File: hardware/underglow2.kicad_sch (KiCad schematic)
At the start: 1 part, among them J101 J_Delphi_Sicma_24

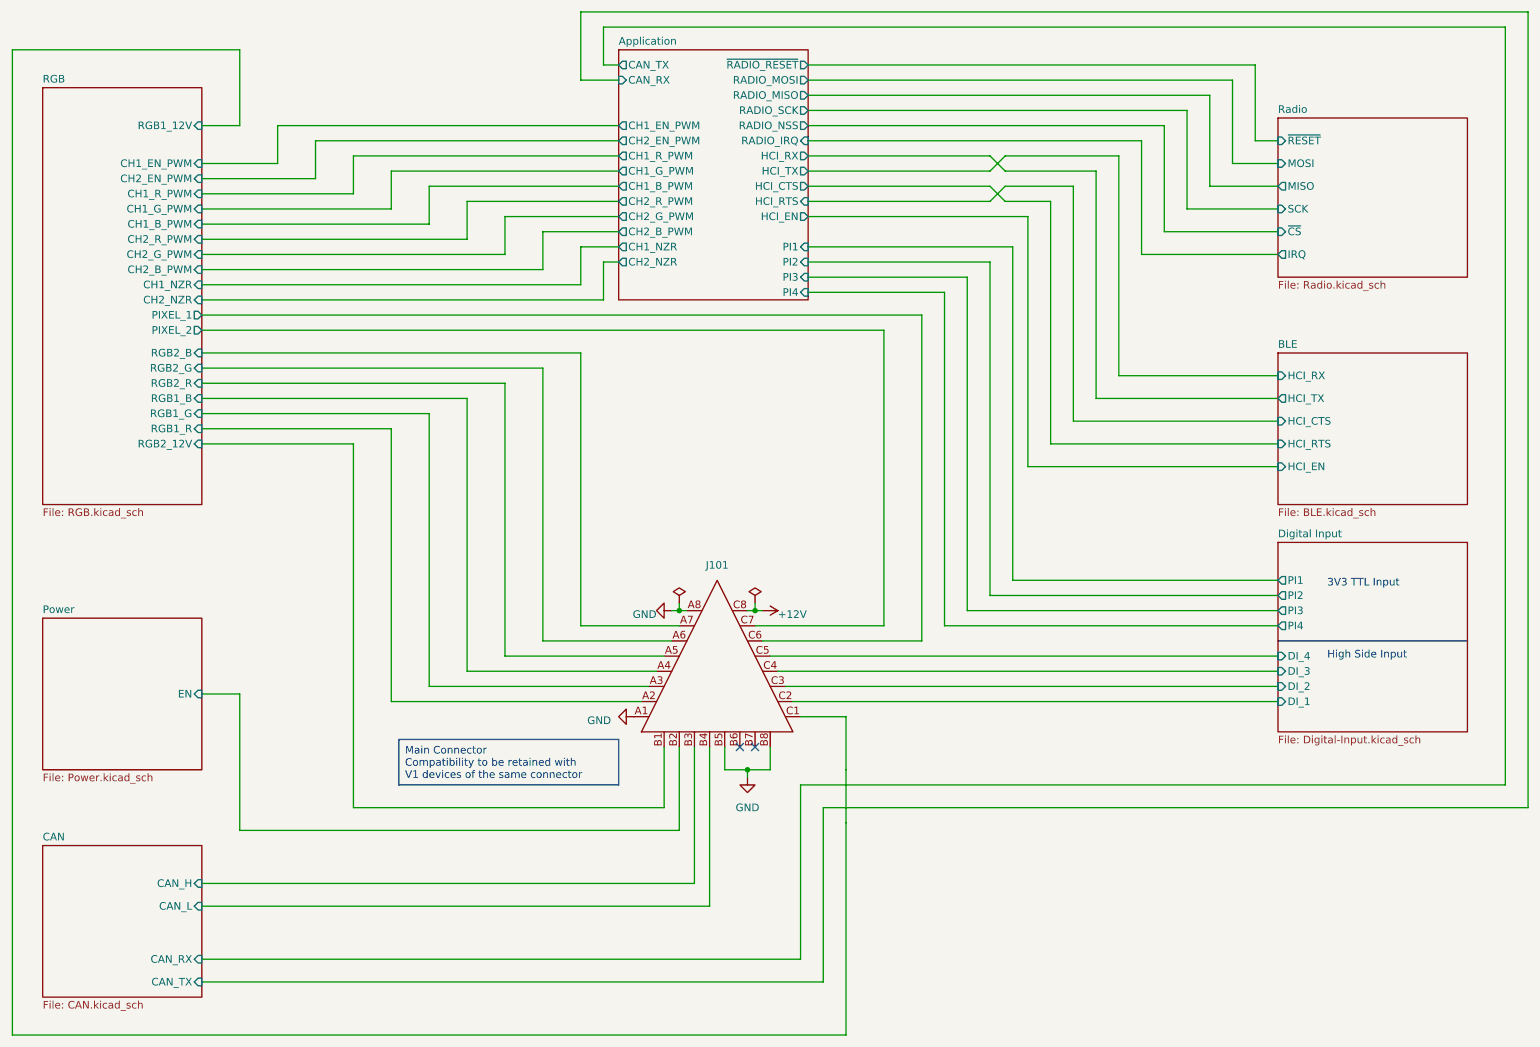
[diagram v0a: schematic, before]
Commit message: ughhhhhhhhhhhhhhhhhhhhhhhhhhhhhhhhhhhhhhhhhhhhhhhhhhh
Signed-off-by: Connor Rigby <connorr@hey.com>
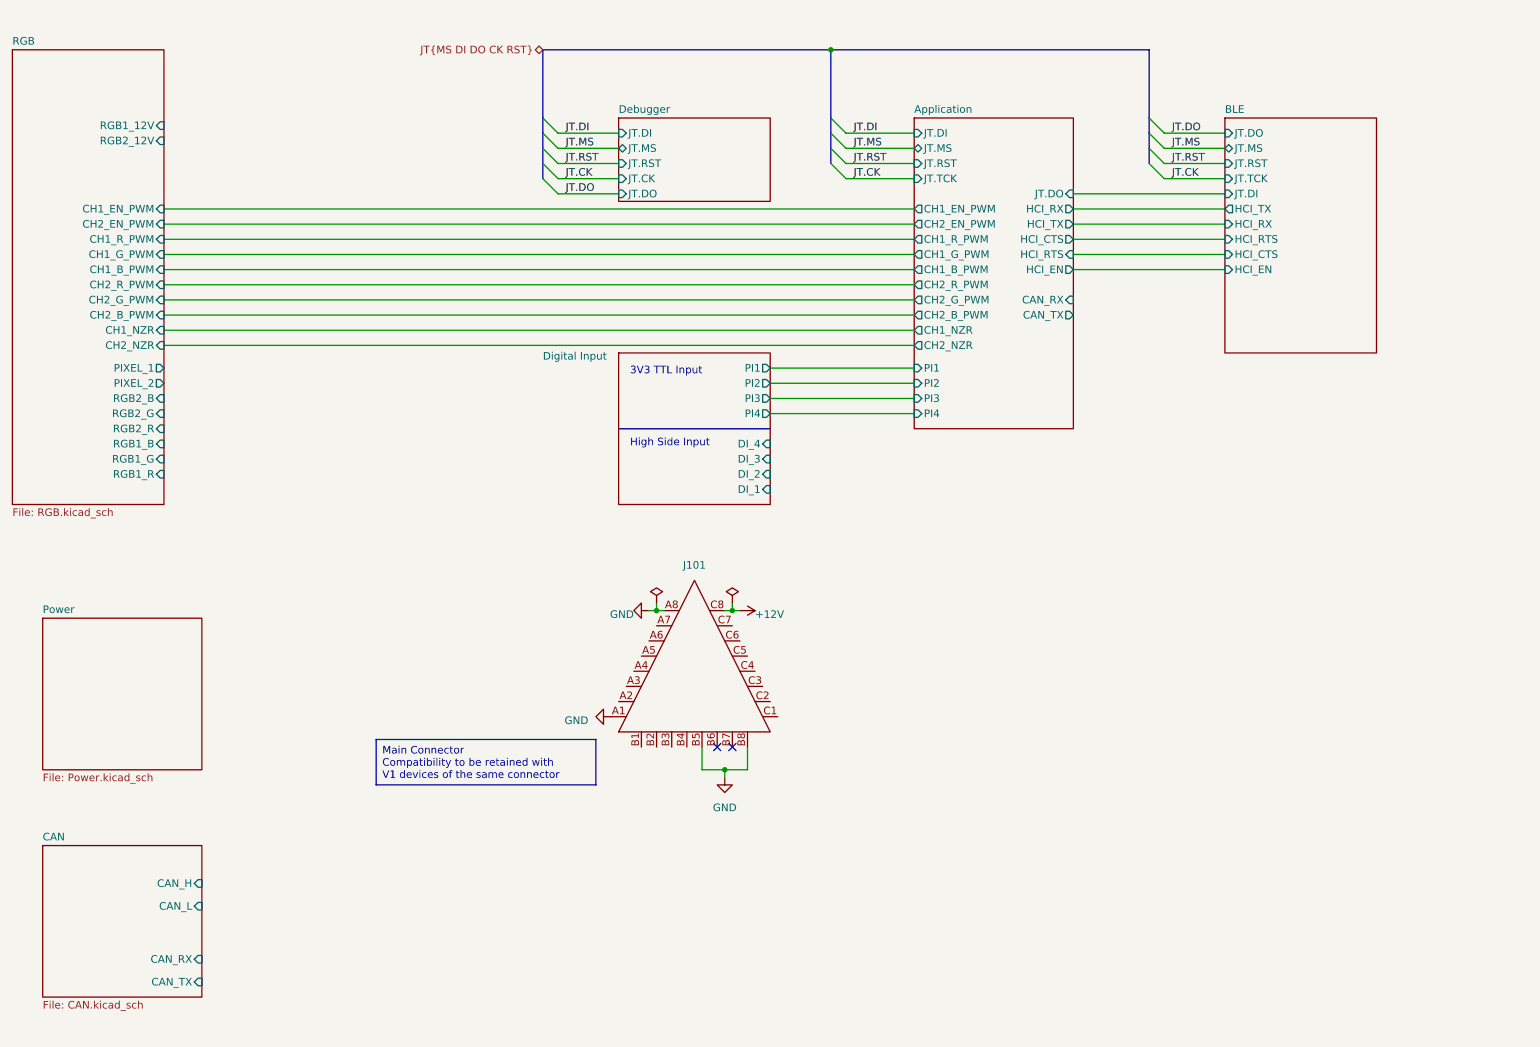
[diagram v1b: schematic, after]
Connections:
- net CAN/CAN_H: no longer J101.B3
- net CAN/CAN_L: no longer J101.B4
- net Digital Input/DI_1: no longer J101.C2
- net Digital Input/DI_2: no longer J101.C3
- net Digital Input/DI_3: no longer J101.C4
- net Digital Input/DI_4: no longer J101.C5
- net RGB/PIXEL_1: no longer J101.C6
- net RGB/PIXEL_2: no longer J101.C7
- net RGB/RGB1_12V: no longer J101.C1
- net RGB/RGB1_B: no longer J101.A4
- net RGB/RGB1_G: no longer J101.A3
- net RGB/RGB1_R: no longer J101.A2
- net RGB/RGB2_12V: no longer J101.B1
- net RGB/RGB2_B: no longer J101.A7
- net RGB/RGB2_G: no longer J101.A6
- net RGB/RGB2_R: no longer J101.A5
- net Power/EN: no longer names the net of J101.B2
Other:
- removed sheet Radio
- added sheet Debugger (Debugger.kicad_sch)
- sheet Application ports: added JT.DI, JT.DO, JT.MS, JT.RST, JT.TCK; removed RADIO_IRQ, RADIO_MISO, RADIO_MOSI, RADIO_NSS, RADIO_SCK, ~{RADIO_RESET}
- sheet BLE ports: added JT.DI, JT.DO, JT.MS, JT.RST, JT.TCK; removed none
- sheet Power ports: added none; removed EN
- moved on the sheet: J101
